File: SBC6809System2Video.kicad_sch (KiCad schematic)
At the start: 68 parts, among them J1 DIN-9, J11 Audio, J2 Conn_Coaxial, U1 IDT7006L35J, U10 74LS157, U11 74LS157, U12 74LS157, U13 74LS157, U14 74LS157, U15 27C64, U16 74LS157, U2 ATF1504AS-xAx44, U3 74LVC1G10, U4 MC68B45, U5 MC68B21, U6 AD725, U7 74HCT393, U8 CD4052B, U9 GAL16V8, Y1 4.433618MHz, Y2 32MHz

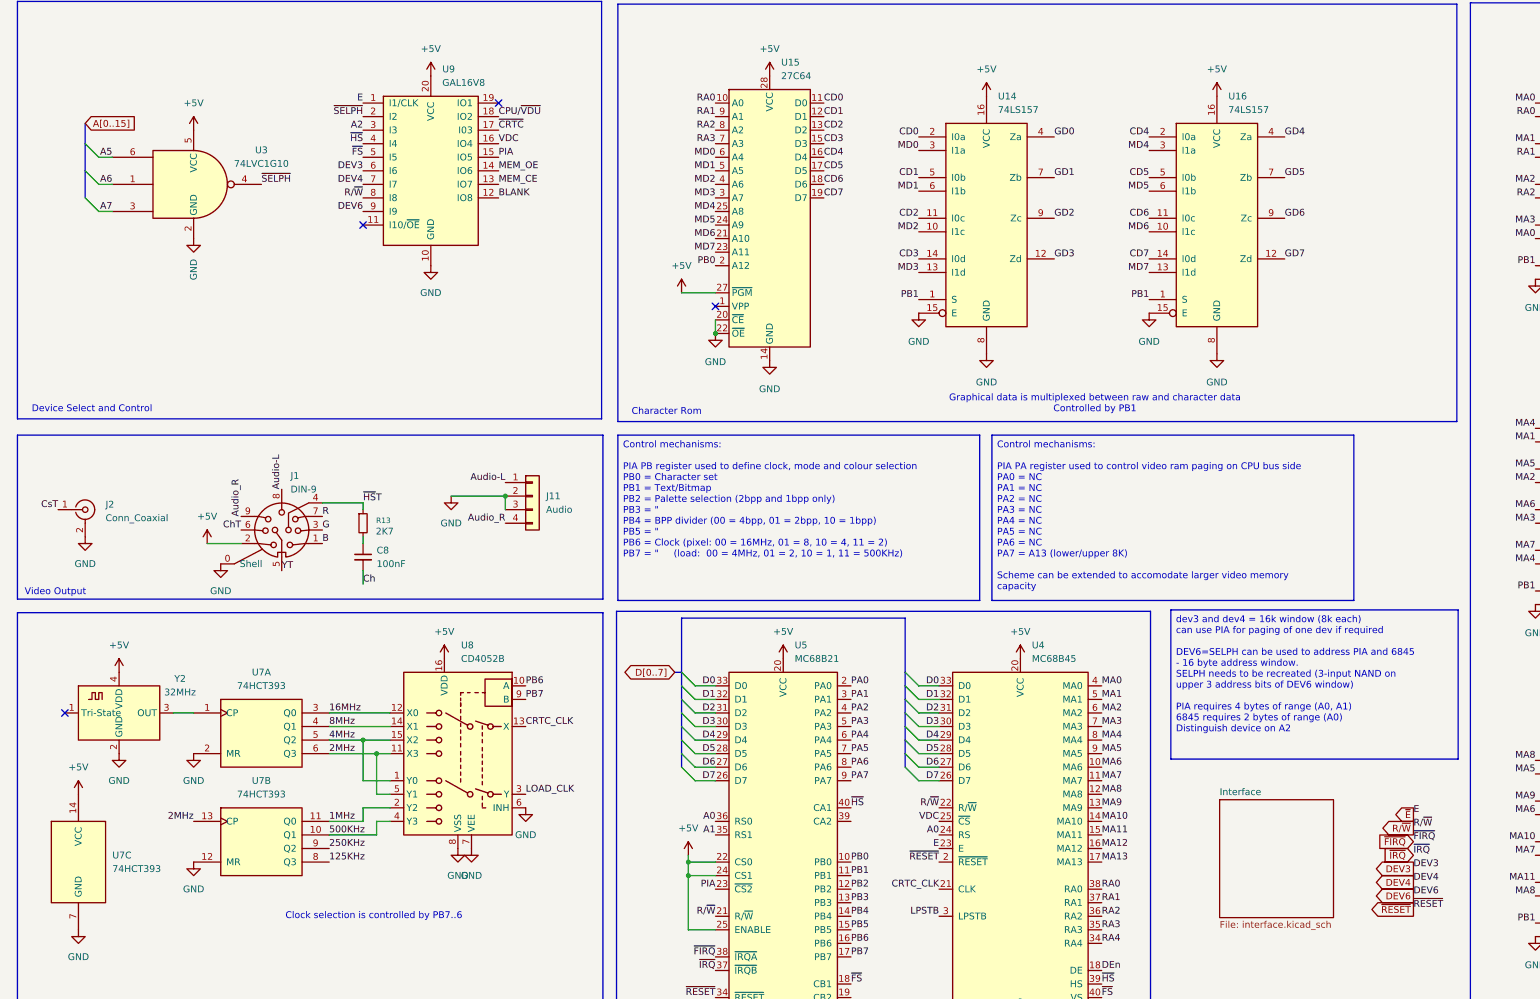
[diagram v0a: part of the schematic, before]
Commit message: convert to dragon
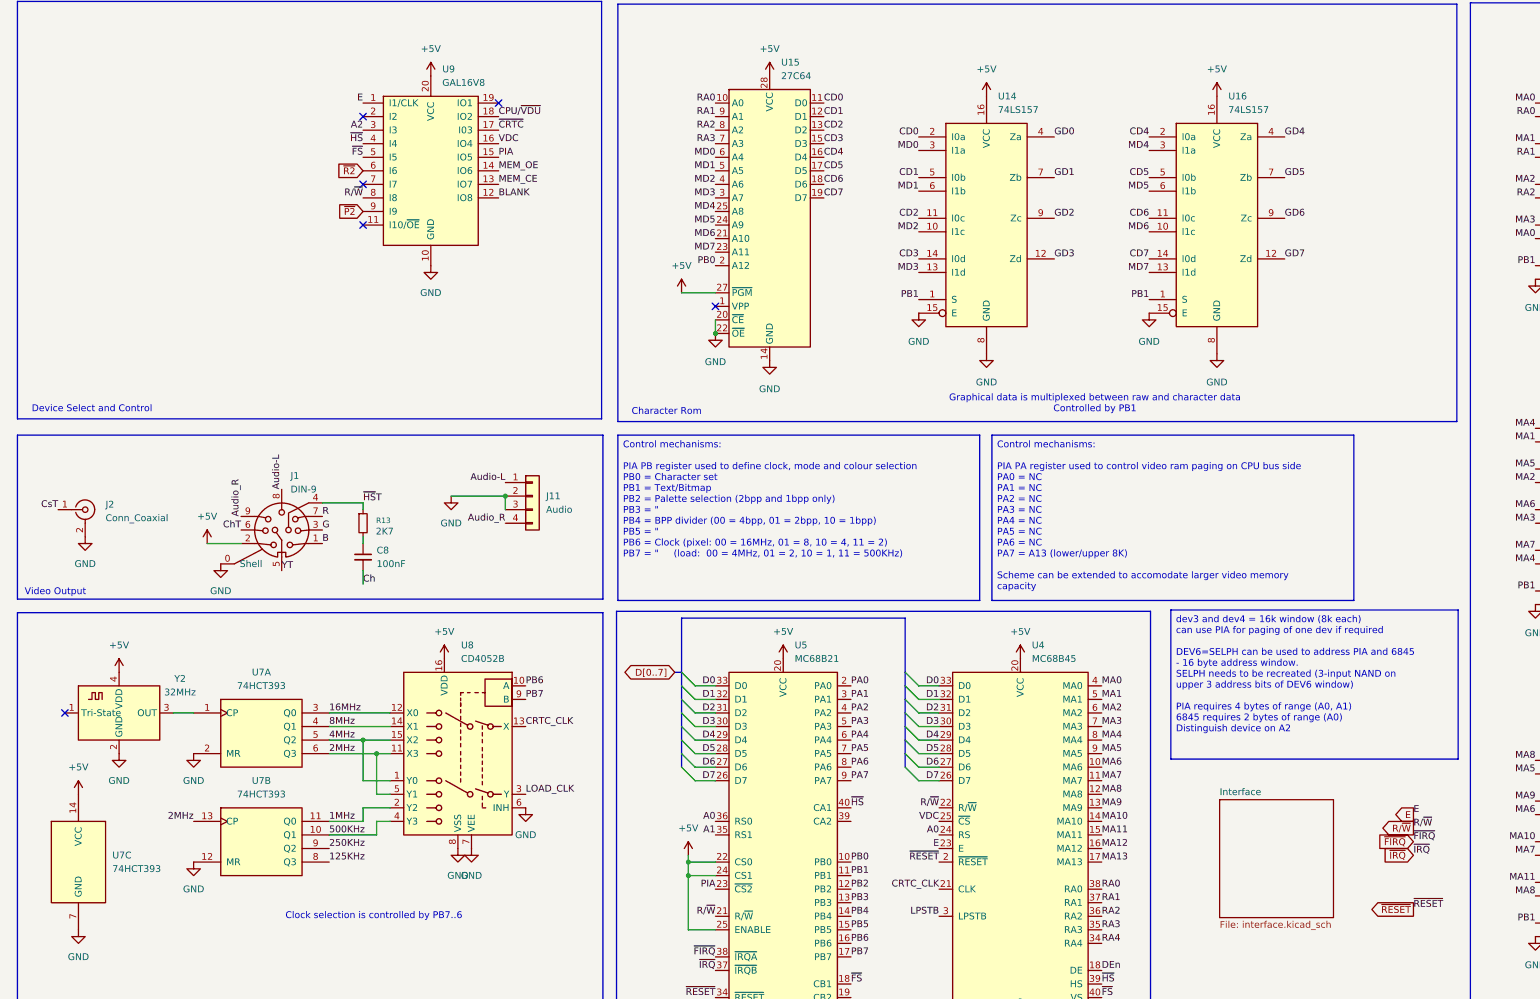
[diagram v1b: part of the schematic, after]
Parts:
- removed U3: 74LVC1G10, PCM_Package_TO_SOT_SMD_AKL:SOT-23-6_Handsoldering, symbol 74xGxx:74LVC1G10
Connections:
- net DEV3 renamed ~{R2}
- net DEV4: no longer names the net of U9.7 (I7)
- net DEV6 renamed ~{P2}
- net ~{E} renamed E
- net ~{SELPH}: no longer names the net of U9.2 (I2)
- no-connect marks 19 -> 21
